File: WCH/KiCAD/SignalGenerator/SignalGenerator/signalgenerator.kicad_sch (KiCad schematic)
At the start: 19 parts, among them J1 Conn_01x10, J2 Conn_01x10, J3 Conn_02x05_Odd_Even, J4 Conn_01x02, J5 Conn_01x07_Pin, SW1 UP, SW2 DOWN, SW3 LEFT, SW4 RIGHT, SW5 ENTER, U1 CH32V003F4P6, U2 AMS1117-3.3, Y1 Crystal_GND24_Small

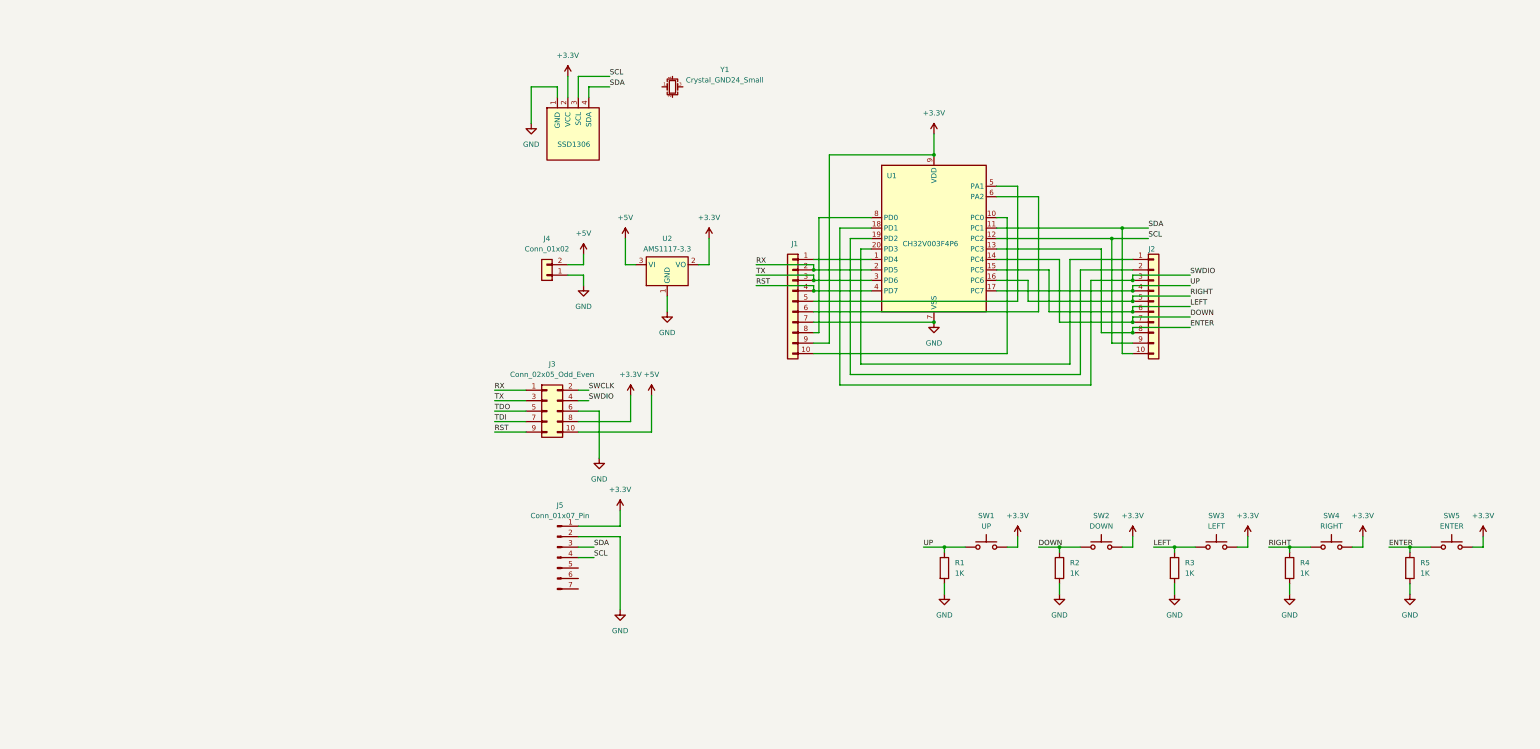
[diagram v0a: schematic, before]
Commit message: New sigal generator board
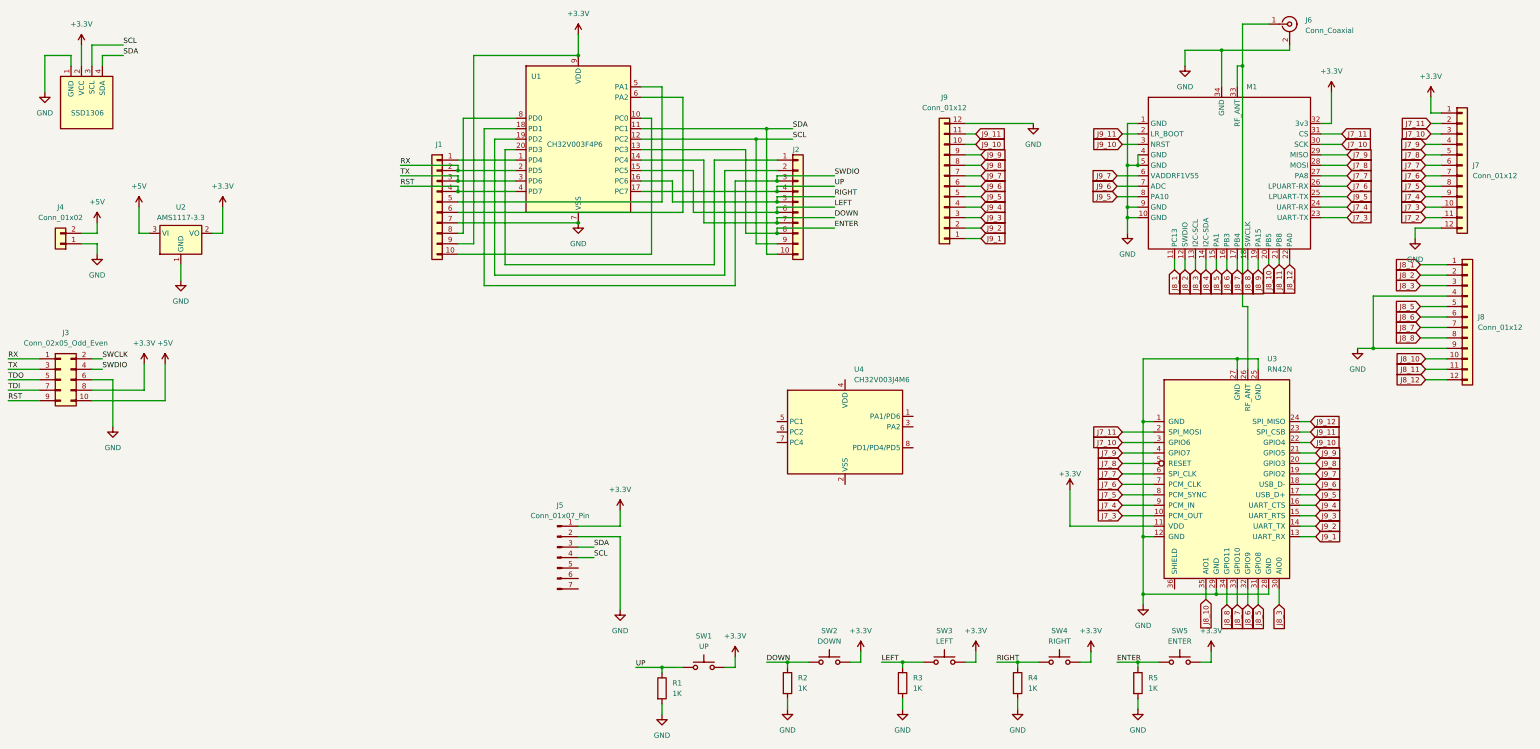
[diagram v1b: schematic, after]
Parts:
- removed Y1: Crystal_GND24_Small, Crystal:Crystal_SMD_0603-4Pin_6.0x3.5mm_HandSoldering, symbol Device:Crystal_GND24_Small
- added J6: Conn_Coaxial, Connector_Coaxial:SMA_Samtec_SMA-J-P-X-ST-EM1_EdgeMount, symbol Connector:Conn_Coaxial
- added J7, J8, J9: Conn_01x12, Connector_PinSocket_2.54mm:PinSocket_1x12_P2.54mm_Vertical, symbol Connector_Generic:Conn_01x12
- added M1: ~, Library:LR1262, symbol wch-mcu:lr1262
- added U3: RN42N, RF_Module:RN42N, symbol RF_Bluetooth:RN42N
- added U4: CH32V003J4M6, Package_SO:SOIC-8_3.9x4.9mm_P1.27mm, symbol wch-mcu:CH32V003J4M6
- J1, J2: footprint Connector_PinHeader_1.27mm:PinHeader_1x10_P1.27mm_Vertical -> Connector_PinHeader_2.00mm:PinHeader_1x10_P2.00mm_Vertical
- SW1, SW2, SW3, SW4, SW5: footprint Button_Switch_THT:SW_PUSH_6mm -> Button_Switch_SMD:SW_Push_1P1T_NO_6x6mm_H9.5mm
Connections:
- net +3.3V: now also J7.1 (Pin_1), M1.32 (3v3), U3.11 (VDD)
- net GND: now also J6.2 (Ext), J7.12 (Pin_12), J8.4 (Pin_4), J8.9 (Pin_9), J9.12 (Pin_12), M1.1 (GND), M1.10 (GND), M1.34 (GND), M1.4 (GND), M1.5 (GND), M1.9 (GND), U3.1 (GND), U3.12 (GND), U3.25 (GND), U3.27 (GND), U3.28 (GND), U3.29 (GND)
- new net: J6.1 (In), M1.33 (RF_ANT), U3.26 (RF_ANT)
- new net J7_10: J7.3 (Pin_3), M1.30 (SCK), U3.3 (GPIO6)
- new net J7_11: J7.2 (Pin_2), M1.31 (CS), U3.2 (SPI_MOSI)
- new net J7_2: J7.11 (Pin_11)
- new net J7_3: J7.10 (Pin_10), M1.23 (UART-TX), U3.10 (PCM_OUT)
- new net J7_4: J7.9 (Pin_9), M1.24 (UART-RX), U3.9 (PCM_IN)
- new net J7_5: J7.8 (Pin_8), U3.8 (PCM_SYNC)
- new net J7_6: J7.7 (Pin_7), M1.26 (LPUART-RX), U3.7 (PCM_CLK)
- new net J7_7: J7.6 (Pin_6), M1.27 (PA8), U3.6 (SPI_CLK)
- new net J7_8: J7.5 (Pin_5), M1.28 (MOSI), U3.5 (RESET)
- new net J7_9: J7.4 (Pin_4), M1.29 (MISO), U3.4 (GPIO7)
- new net J8_1: J8.1 (Pin_1), M1.11 (PC13)
- new net J8_10: J8.10 (Pin_10), M1.20 (PB5), U3.35 (AIO1)
- new net J8_11: J8.11 (Pin_11), M1.21 (PB8)
- new net J8_12: J8.12 (Pin_12), M1.22 (PA0)
- new net J8_2: J8.2 (Pin_2), M1.12 (SWDIO)
- new net J8_3: J8.3 (Pin_3), M1.13 (I2C-SCL), U3.30 (AIO0)
- new net J8_4: M1.14 (I2C-SDA)
- new net J8_5: J8.5 (Pin_5), M1.15 (PA1), U3.31 (GPIO8)
- new net J8_6: J8.6 (Pin_6), M1.16 (PB3), U3.32 (GPIO9)
- new net J8_7: J8.7 (Pin_7), M1.17 (PB4), U3.33 (GPIO10)
- new net J8_8: J8.8 (Pin_8), M1.18 (SWCLK), U3.34 (GPIO11)
- new net J8_9: M1.19 (PA15)
- new net J9_1: J9.1 (Pin_1), U3.13 (UART_RX)
- new net J9_10: J9.10 (Pin_10), M1.3 (NRST), U3.22 (GPIO4)
- new net J9_11: J9.11 (Pin_11), M1.2 (LR_BOOT), U3.23 (SPI_CSB)
- new net J9_12: U3.24 (SPI_MISO)
- new net J9_2: J9.2 (Pin_2), U3.14 (UART_TX)
- new net J9_3: J9.3 (Pin_3), U3.15 (UART_RTS)
- new net J9_4: J9.4 (Pin_4), U3.16 (UART_CTS)
- new net J9_5: J9.5 (Pin_5), M1.25 (LPUART-TX), M1.8 (PA10), U3.17 (USB_D+)
- new net J9_6: J9.6 (Pin_6), M1.7 (ADC), U3.18 (USB_D-)
- new net J9_7: J9.7 (Pin_7), M1.6 (VADDRF1V55), U3.19 (GPIO2)
- new net J9_8: J9.8 (Pin_8), U3.20 (GPIO3)
- new net J9_9: J9.9 (Pin_9), U3.21 (GPIO5)
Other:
- moved on the sheet: J1, J2, J3, J4, R1, R2, R3, R4, R5, SW1, SW2, SW3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

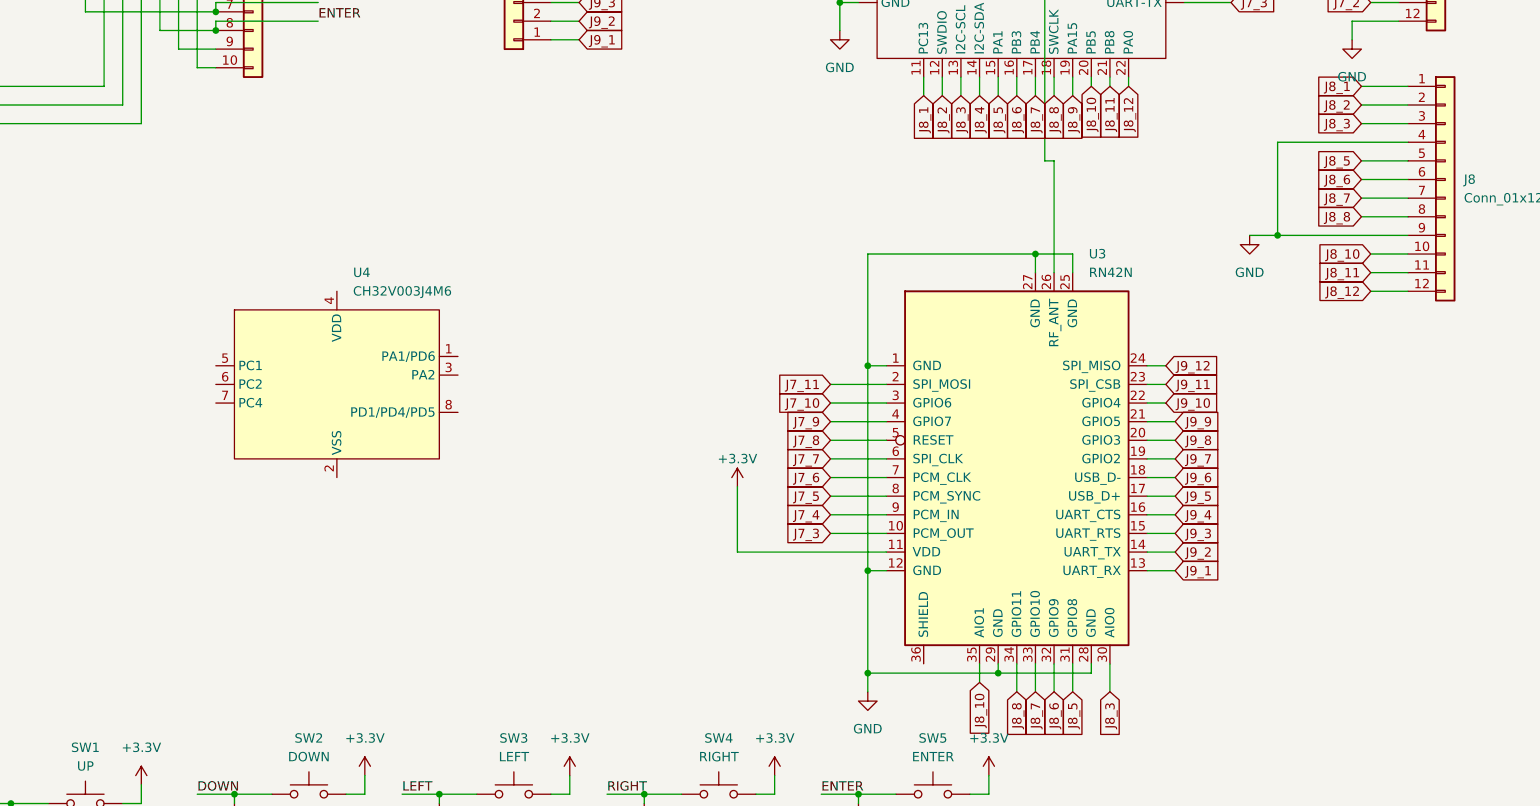
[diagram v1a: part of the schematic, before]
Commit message: PCB
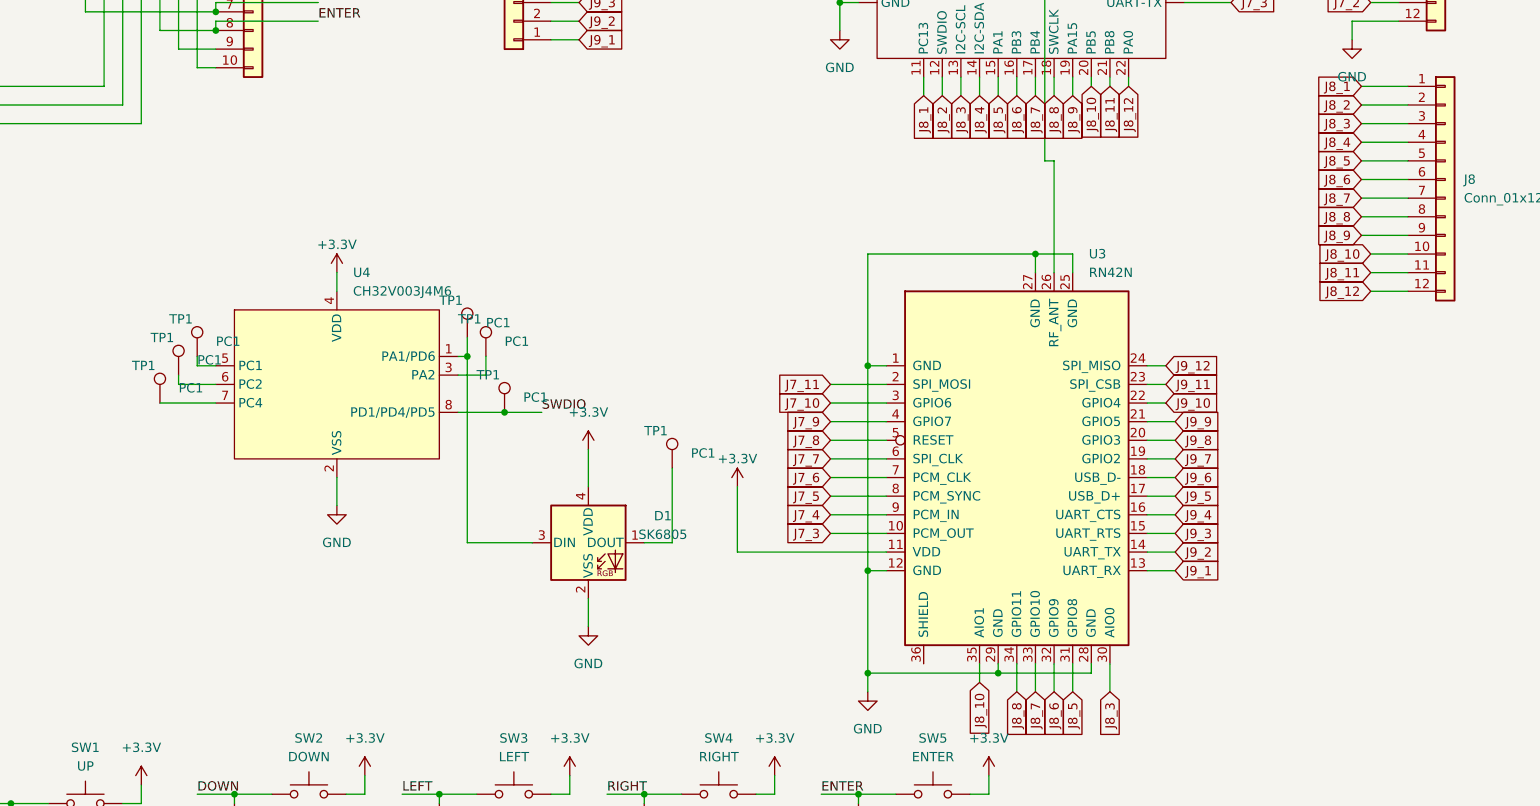
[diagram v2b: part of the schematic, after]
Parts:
- added D1: SK6805, LED_SMD:LED_SK6812_EC15_1.5x1.5mm, symbol LED:SK6805
- added TP1 (x7): PC1, TestPoint:TestPoint_Pad_D2.0mm, symbol Connector:TestPoint
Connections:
- net +3.3V: now also U4.4 (VDD), D1.4 (VDD)
- net GND: now also U4.2 (VSS), D1.2 (VSS); no longer J8.4 (Pin_4), J8.9 (Pin_9)
- net J8_4: now also J8.4 (Pin_4)
- net J8_9: now also J8.9 (Pin_9)
- net SWDIO: now also U4.8 (PD1/PD4/PD5), TP1.1
- net at U4.1 (PA1/PD6): now also D1.3 (DIN), TP1.1
- net at U4.3 (PA2): now also TP1.1
- net at U4.5 (PC1): now also TP1.1
- net at U4.6 (PC2): now also TP1.1
- net at U4.7 (PC4): now also TP1.1
- new net: D1.1 (DOUT), TP1.1
